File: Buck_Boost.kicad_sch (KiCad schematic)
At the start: 4 parts, among them U7 TPS63001DRC

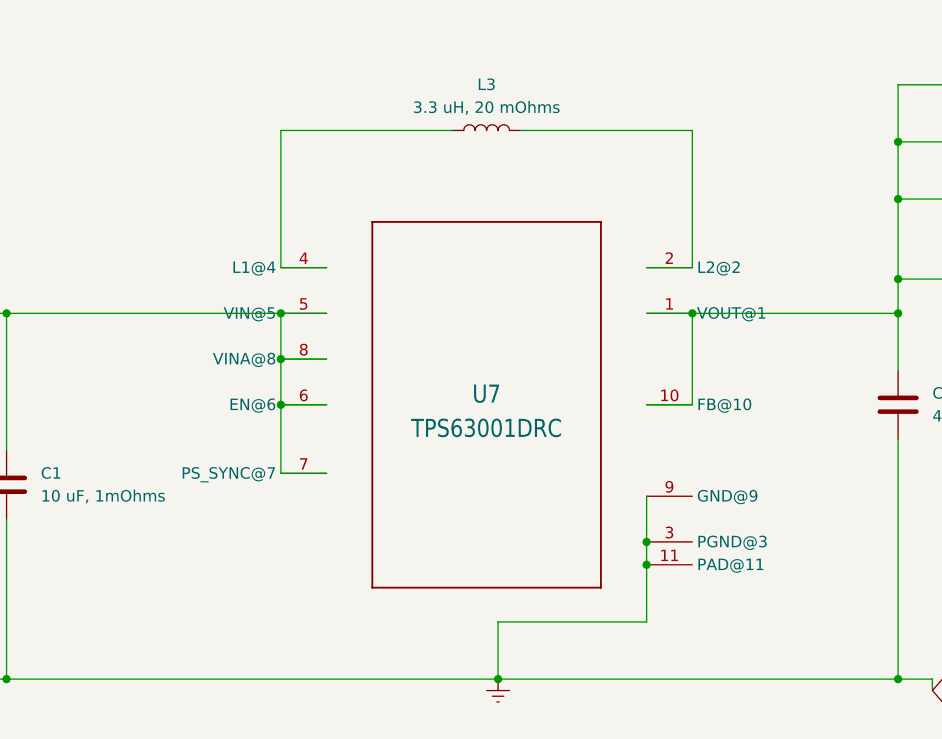
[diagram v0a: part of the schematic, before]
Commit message: Add files via upload
Finished the main schematic as well as the sub schematics
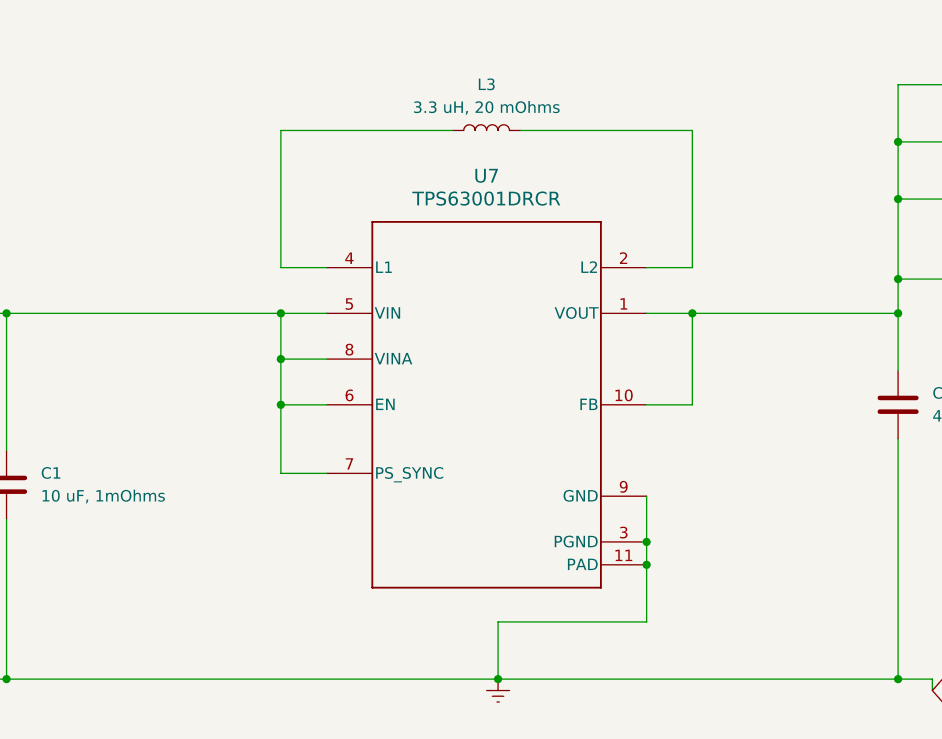
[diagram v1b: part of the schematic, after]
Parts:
- removed U7: TPS63001DRC, Buck-Boost Converter Chip:DRC0010J, symbol 2024-09-27_13-12-33-eagle-import:TPS63001DRCRTPS63001DRCR
- added U7: TPS63001DRCR, Buck-Boost:DRC0010J, symbol Buck-Boost Chip:TPS63001DRCR
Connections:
- net Battery Box Vout (Flyback Diode): now also U7.5 (VIN), U7.6 (EN), U7.7 (PS_SYNC), U7.8 (VINA)
- net Earth: now also U7.11 (PAD), U7.3 (PGND), U7.9 (GND)
- net GPS Pin Four (Vbackup): now also U7.1 (VOUT), U7.10 (FB)
- net at L3.2: now also U7.2 (L2)
- net at L3.1: now also U7.4 (L1)
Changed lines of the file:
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@@
+	)
+	(junction
+		(at 128.27 115.57)
+		(diameter 0)
+		(color 0 0 0 0)
+	)
+	(junction
+		(at 111.76 130.81)
+		(diameter 0)
+		(color 0 0 0 0)
 	)
 	(junction
@@
 	)
 	(junction
-		(at 111.76 130.81)
-		(diameter 0)
-		(color 0 0 0 0)
-	)
-	(junction
-		(at 128.27 115.57)
-		(diameter 0)
-		(color 0 0 0 0)
-	)
-	(junction
 		(at 156.21 86.36)
 		(diameter 0)
@@
 	(wire
 		(pts
+			(xy 128.27 115.57) (xy 128.27 118.11)
+		)
+		(stroke
+			(width 0)
+			(type default)
+		)
+	)
+	(wire
+		(pts
 			(xy 156.21 130.81) (xy 111.76 130.81)
 		)
@@
 	(wire
 		(pts
-			(xy 128.27 115.57) (xy 128.27 118.11)
-		)
-		(stroke
-			(width 0)
-			(type default)
-		)
-	)
-	(wire
-		(pts
 			(xy 57.15 105.41) (xy 57.15 90.17)
 		)
@@
 	(wire
 		(pts
+			(xy 87.63 95.25) (xy 87.63 100.33)
+		)
+		(stroke
+			(width 0)
+			(type default)
+		)
+	)
+	(wire
+		(pts
+			(xy 57.15 90.17) (xy 87.63 90.17)
+		)
+		(stroke
+			(width 0)
+			(type default)
+		)
+	)
+	(wire
+		(pts
+			(xy 156.21 71.12) (xy 156.21 64.77)
+		)
+		(stroke
+			(width 0)
+			(type default)
+		)
+	)
+	(wire
+		(pts
+			(xy 87.63 100.33) (xy 92.71 100.33)
+		)
+		(stroke
+			(width 0)
+			(type default)
+		)
+	)
+	(wire
+		(pts
+			(xy 36.83 86.36) (xy 36.83 90.17)
+		)
+		(stroke
+			(width 0)
+			(type default)
+		)
+	)
+	(wire
+		(pts
 			(xy 128.27 118.11) (xy 128.27 124.46)
-		)
-		(stroke
-			(width 0)
-			(type default)
-		)
-	)
-	(wire
-		(pts
-			(xy 87.63 95.25) (xy 87.63 100.33)
-		)
-		(stroke
-			(width 0)
-			(type default)
-		)
-	)
-	(wire
-		(pts
-			(xy 57.15 90.17) (xy 87.63 90.17)
-		)
-		(stroke
-			(width 0)
-			(type default)
-		)
-	)
-	(wire
-		(pts
-			(xy 156.21 71.12) (xy 156.21 64.77)
-		)
-		(stroke
-			(width 0)
-			(type default)
-		)
-	)
-	(wire
-		(pts
-			(xy 87.63 100.33) (xy 92.71 100.33)
-		)
-		(stroke
-			(width 0)
-			(type default)
-		)
-	)
-	(wire
-		(pts
-			(xy 36.83 86.36) (xy 36.83 90.17)
 		)
 		(stroke
@@
 				(path "/eb9a8801-b205-4599-90e8-b0089b4de1f9/d1b18d40-22b1-4c43-a62b-141a1593bdb1"
 					(reference "#PWR07")
-					(unit 1)
-				)
-			)
-		)
-	)
-	(symbol
-		(lib_id "2024-09-27_13-12-33-eagle-import:TPS63001DRCRTPS63001DRCR")
-		(at 110.49 100.33 0)
-		(unit 1)
-		(exclude_from_sim no)
-		(in_bom yes)
-		(on_board yes)
-		(dnp no)
-		(property "Reference" "U7"
-			(at 110.49 100.33 0)
-			(effects
-				(font
-					(size 2 1.7)
-				)
-				(justify bottom)
-			)
-		)
-		(property "Value" "TPS63001DRC"
-			(at 110.49 104.14 0)
-			(effects
-				(font
-					(size 2 1.7)
-				)
-				(justify bottom)
-			)
-		)
-		(property "Footprint" "Buck-Boost Converter Chip:DRC0010J"
-			(at 110.49 100.33 0)
-			(effects
-				(font
-					(size 1.27 1.27)
-				)
-				(hide yes)
-			)
-		)
-		(property "Datasheet" ""
-			(at 110.49 100.33 0)
-			(effects
-				(font
-					(size 1.27 1.27)
-				)
-				(hide yes)
-			)
-		)
-		(property "Description" ""
-			(at 110.49 100.33 0)
-			(effects
-				(font
-					(size 1.27 1.27)
-				)
-				(hide yes)
-			)
-		)
-		(pin "1"
-		)
-		(pin "10"
-		)
-		(pin "11"
-		)
-		(pin "2"
-		)
-		(pin "3"
-		)
-		(pin "4"
-		)
-		(pin "5"
-		)
-		(pin "6"
-		)
-		(pin "7"
-		)
-		(pin "8"
-		)
-		(pin "9"
-		)
-		(instances
-			(project "PCB desing"
-				(path "/eb9a8801-b205-4599-90e8-b0089b4de1f9/d1b18d40-22b1-4c43-a62b-141a1593bdb1"
-					(reference "U7")
 					(unit 1)
 				)
@@
 					(unit 1)
 				)
+			)
+		)
+	)
+	(symbol
+		(lib_id "Buck-Boost Chip:TPS63001DRCR")
+		(at 110.49 100.33 0)
+		(unit 1)
+		(exclude_from_sim no)
+		(in_bom yes)
+		(on_board yes)
+		(dnp no)
+		(fields_autoplaced yes)
+		(property "Reference" "U7"
+			(at 110.49 74.93 0)
+			(effects
+				(font
+					(size 1.524 1.524)
+				)
+			)
+		)
+		(property "Value" "TPS63001DRCR"
+			(at 110.49 77.47 0)
+			(effects
+				(font
+					(size 1.524 1.524)
+				)
+			)
+		)
+		(property "Footprint" "Buck-Boost:DRC0010J"
+			(at 110.49 100.33 0)
+			(effects
+				(font
+					(size 1.27 1.27)
+					(italic yes)
+				)
+				(hide yes)
+			)
+		)
+		(property "Datasheet" "TPS63001DRCR"
+			(at 110.49 100.33 0)
+			(effects
+				(font
+					(size 1.27 1.27)
+					(italic yes)
+				)
+				(hide yes)
+			)
+		)
+		(property "Description" ""
+			(at 110.49 100.33 0)
+			(effects
+				(font
+					(size 1.27 1.27)
+				)
+				(hide yes)
+			)
+		)
+		(pin "11"
+		)
+		(pin "9"
+		)
+		(pin "8"
+		)
+		(pin "3"
+		)
+		(pin "2"
+		)
+		(pin "6"
+		)
+		(pin "5"
+		)
+		(pin "4"
+		)
+		(pin "10"
+		)
+		(pin "7"
+		)
+		(pin "1"
+		)
+		(instances
+			(project "PCB desing"
+				(path "/eb9a8801-b205-4599-90e8-b0089b4de1f9/d1b18d40-22b1-4c43-a62b-141a1593bdb1"
+					(reference "U7")
+					(unit 1)
+				)
